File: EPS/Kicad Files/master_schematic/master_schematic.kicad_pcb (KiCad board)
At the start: 2 copper layers, 96 x 90 mm, 79 parts, among them J1 USB_C_Receptacle, J2 436500212, J3 Conn_02x20_Odd_Even, J4 Conn_01x05_Female, Q1 FZT688BTA, Q2 FZT688BTA, U1 RPM5.0-2.0, U2 RPM5.0-2.0, U3 RPM3.3-2.0, U4 INA3221, U5 MAX77757JEFG435+, U6 MAX17055EWL+T, U7 ATA6560-GAQW-VAO, U8 PIC18F27Q84-E/SP

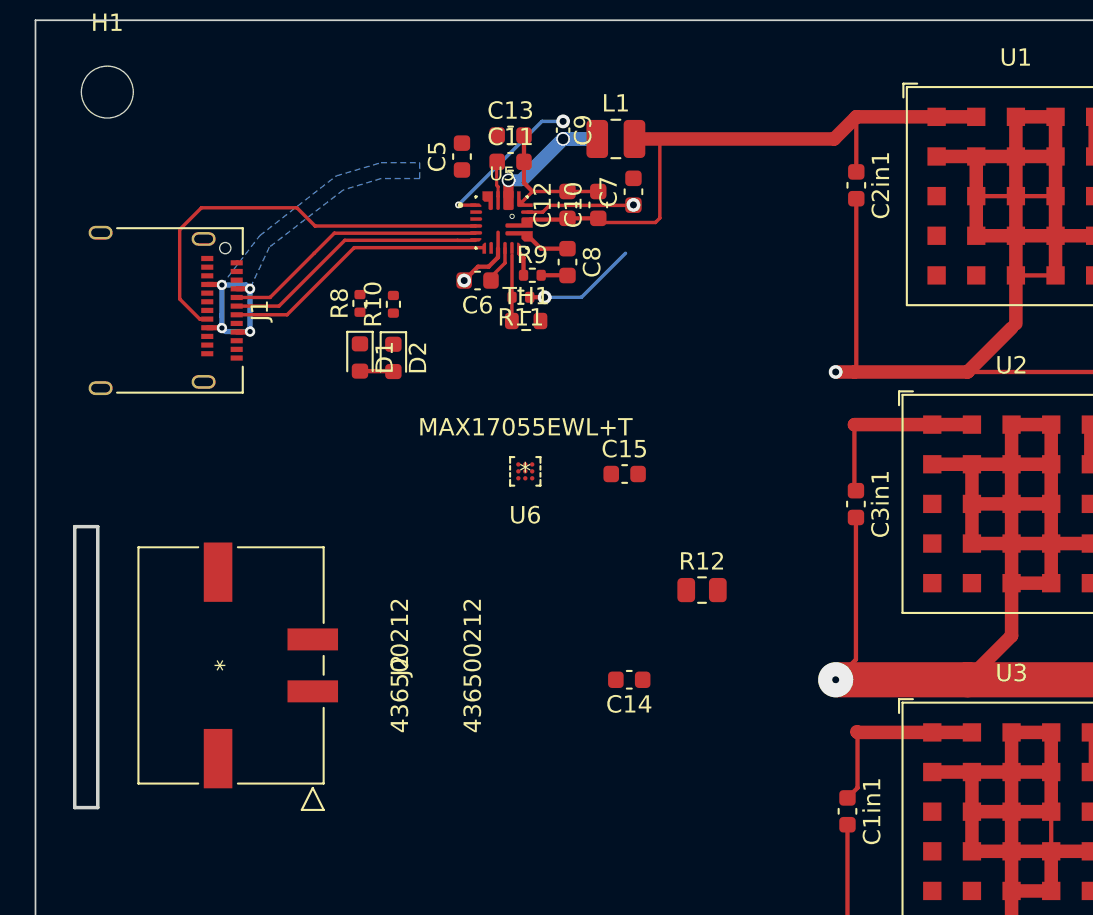
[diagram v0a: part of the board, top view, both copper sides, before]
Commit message: eps updated
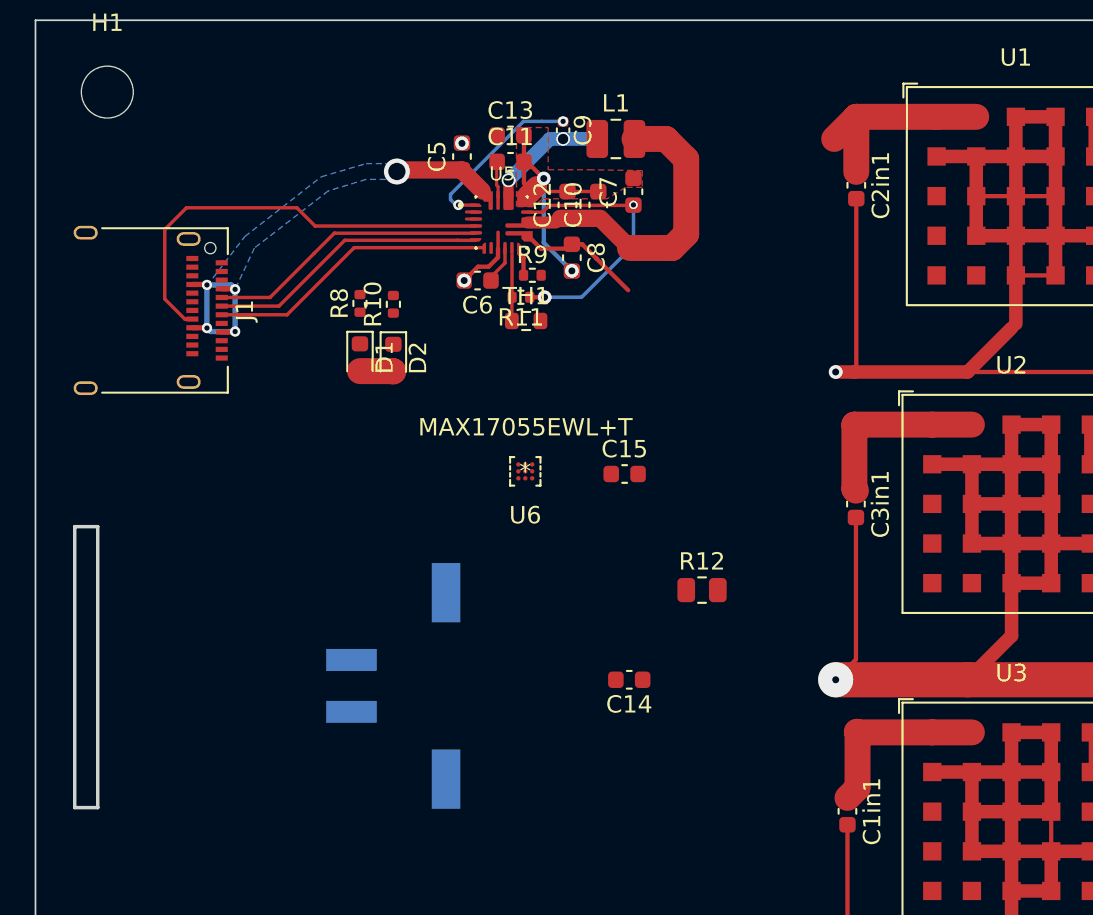
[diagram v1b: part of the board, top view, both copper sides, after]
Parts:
- J2: moved to B.Cu
- moved J2 12.5 mm to (61.0, 94.3)
- moved J1 0.86 mm to (43.3, 72.6)
- moved C8 0.36 mm to (68.6, 69.6)
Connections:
- R9 pad 2: GNDPWR -> GND
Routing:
- net /charge schem/SYSPOWER: track 60.6 -> 53.3 mm
- net GNDPWR: track 9.57 -> 15.6 mm, vias 0 -> 2
- net Net-(C5-Pad1): track 11.7 -> 17.1 mm, vias 4 -> 5
- net /charge schem/V_BAT: track 2.60 -> 6.96 mm
- net Net-(C7-Pad1): track 12.9 -> 15.9 mm
- net Net-(C9-Pad1): track 9.07 -> 10.2 mm
- net Net-(J1-PadB5): track 24.1 -> 25.0 mm
- net Net-(J1-PadA7): track 15.9 -> 16.7 mm
- net Net-(J1-PadA6): track 15.4 -> 16.2 mm
- net Net-(J1-PadA5): track 15.3 -> 16.2 mm
- net Net-(R8-Pad2): track 0.00 -> 0.56 mm
- net Net-(R10-Pad2): track 0.00 -> 0.56 mm
- net GND: vias 10 -> 11
- net (no net): vias 1 -> 0
- added copper zone on F.Cu, net GNDPWR
